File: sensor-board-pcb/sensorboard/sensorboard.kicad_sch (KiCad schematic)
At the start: 138 parts, among them J1 TO_MOTHERBOARD_JACK, J10 PZT_008, J100 PZT_098, J101 PZT_099, J102 PZT_100, J103 PZT_101, J104 PZT_102, J105 PZT_103, J106 PZT_104, J107 PZT_105, J108 PZT_106, J109 PZT_107, J11 PZT_009, J110 PZT_108, J111 PZT_109, J112 PZT_110, J113 PZT_111, J114 PZT_112, J115 PZT_113, J116 PZT_114, J117 PZT_115, J118 PZT_116, J119 PZT_117, J12 PZT_010, J120 PZT_118, J121 PZT_119, J122 PZT_120, J123 PZT_121, J124 PZT_122, J125 PZT_123, J126 PZT_124, J127 PZT_125, J128 PZT_126, J129 PZT_127, J13 PZT_011, J14 PZT_012, J15 PZT_013, J16 PZT_014, J17 PZT_015, J18 PZT_016, J19 PZT_017, J2 PZT_000, J20 PZT_018, J21 PZT_019, J22 PZT_020, J23 PZT_021, J24 PZT_022, J25 PZT_023, J26 PZT_024, J27 PZT_025, J28 PZT_026, J29 PZT_027, J3 PZT_001, J30 PZT_028, J31 PZT_029, J32 PZT_030, J33 PZT_031, J34 PZT_032, J35 PZT_033, J36 PZT_034, J37 PZT_035, J38 PZT_036, J39 PZT_037, J4 PZT_002, J40 PZT_038, J41 PZT_039, J42 PZT_040, J43 PZT_041, J44 PZT_042, J45 PZT_043, J46 PZT_044, J47 PZT_045, J48 PZT_046, J49 PZT_047, J5 PZT_003, J50 PZT_048, J51 PZT_049, J52 PZT_050, J53 PZT_051, J54 PZT_052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

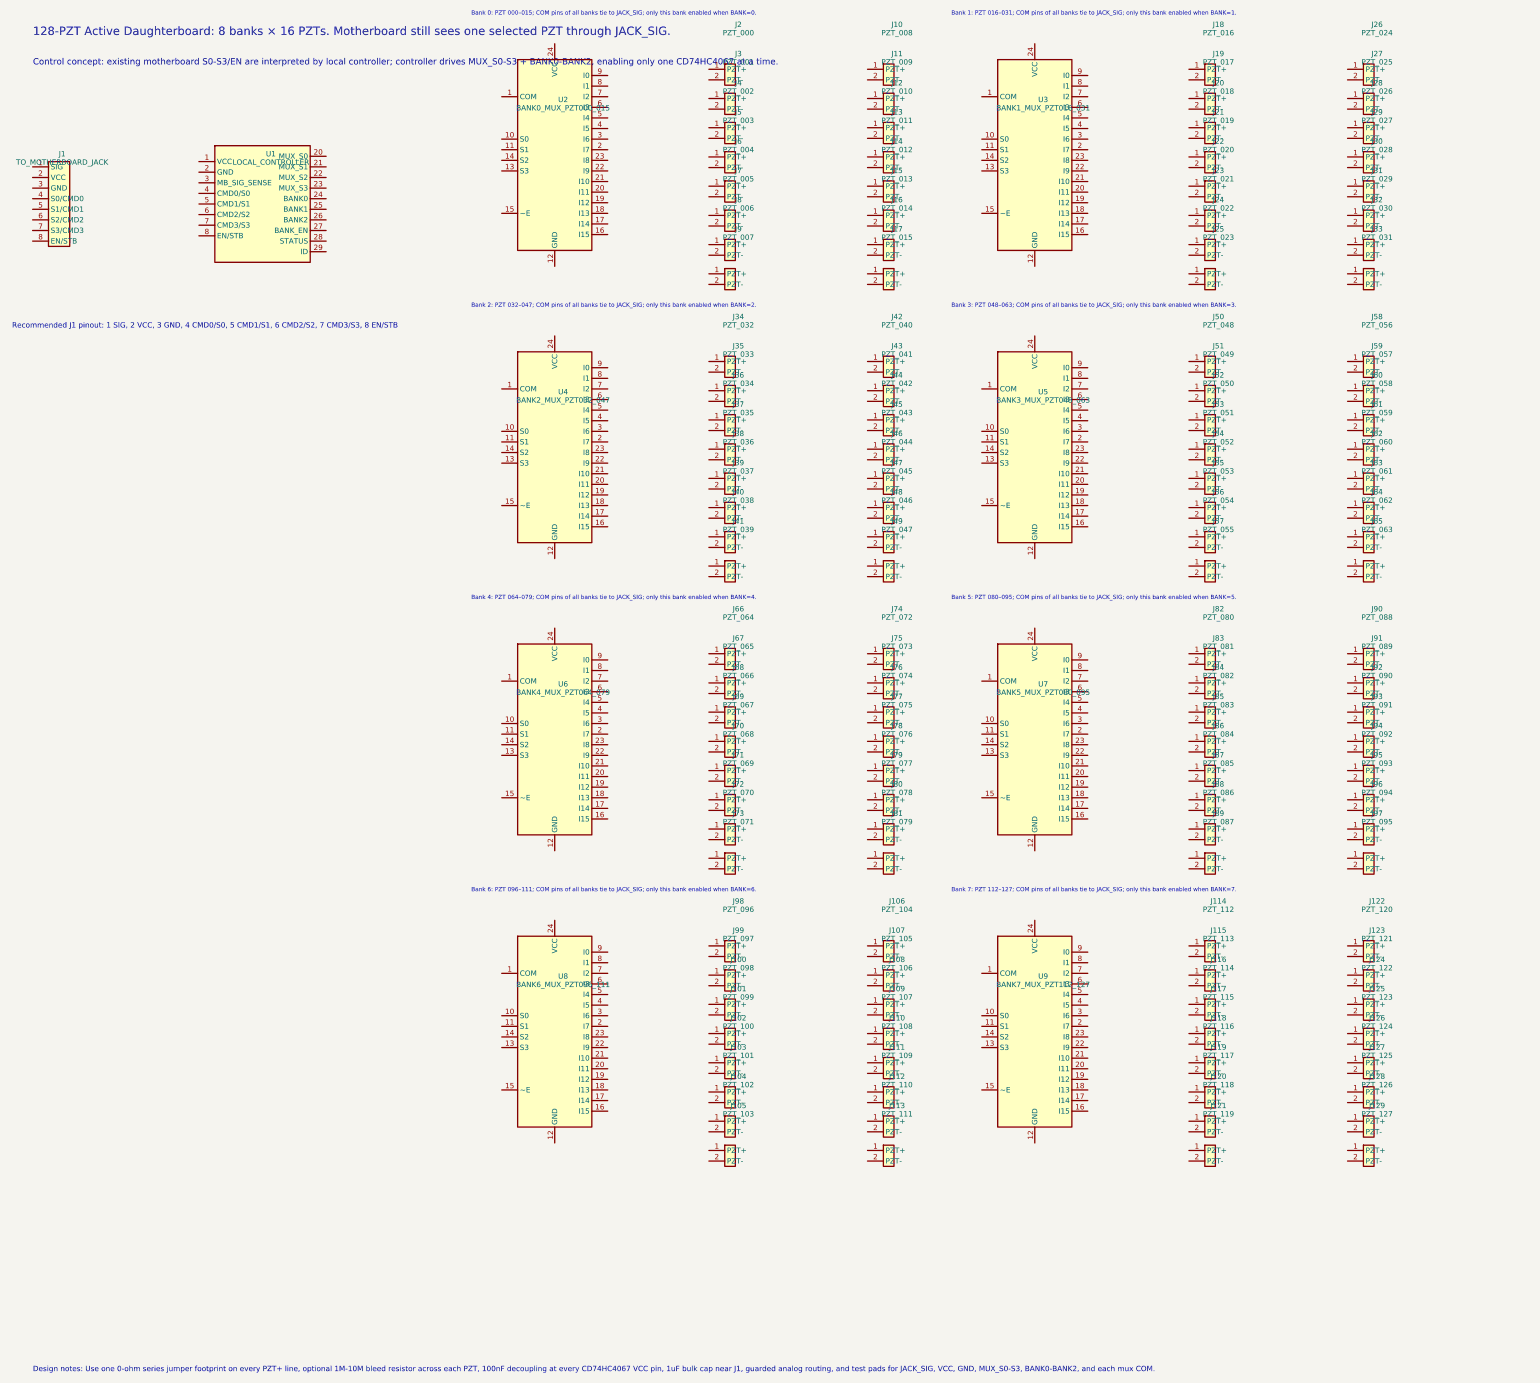
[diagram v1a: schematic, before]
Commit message: fix schem
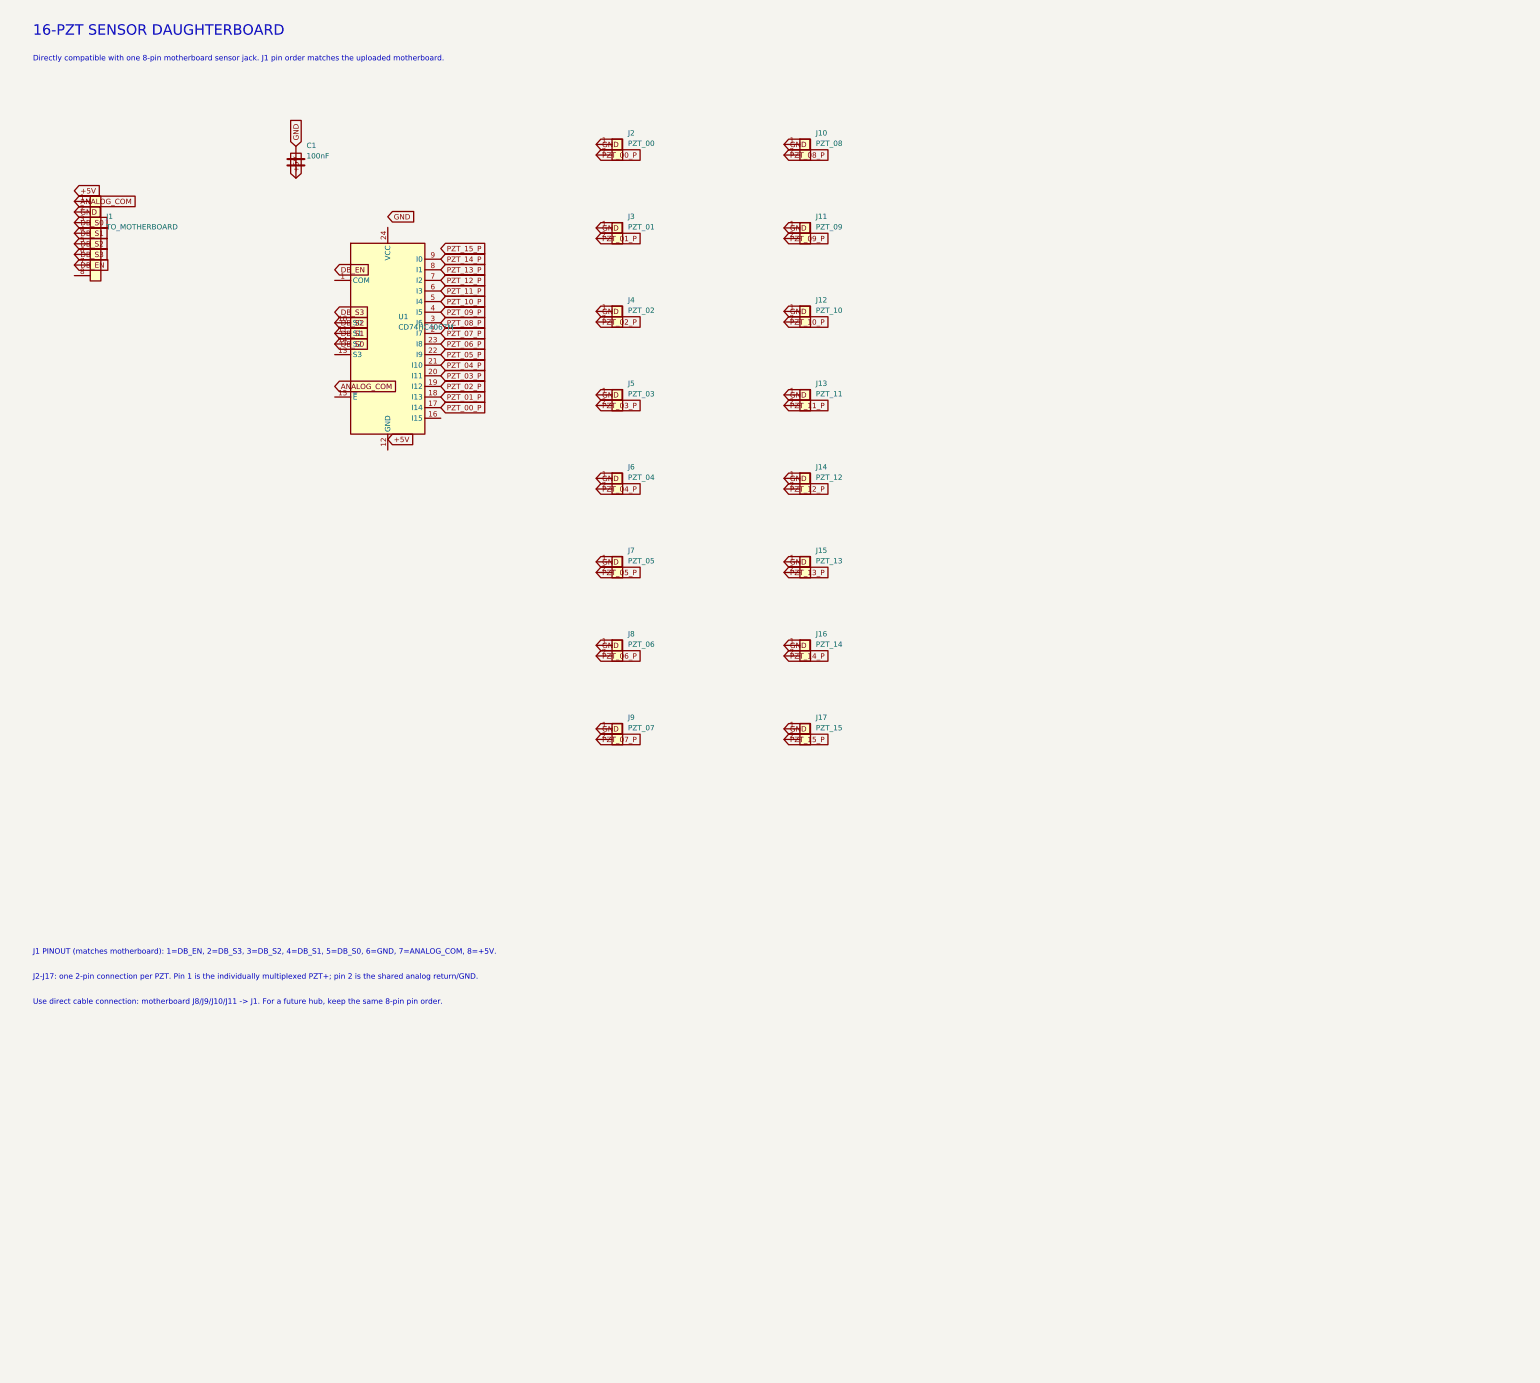
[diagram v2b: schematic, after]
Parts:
- removed J1: TO_MOTHERBOARD_JACK, Connector_PinHeader_2.54mm:PinHeader_1x08_P2.54mm_Vertical, symbol Daughter:MicroFit_01x08_Motherboard
- removed J10: PZT_008, Connector_PinHeader_2.54mm:PinHeader_1x02_P2.54mm_Vertical, symbol Daughter:PZT_Conn_01x02
- removed J100: PZT_098, Connector_PinHeader_2.54mm:PinHeader_1x02_P2.54mm_Vertical, symbol Daughter:PZT_Conn_01x02
- removed J101: PZT_099, Connector_PinHeader_2.54mm:PinHeader_1x02_P2.54mm_Vertical, symbol Daughter:PZT_Conn_01x02
- removed J102: PZT_100, Connector_PinHeader_2.54mm:PinHeader_1x02_P2.54mm_Vertical, symbol Daughter:PZT_Conn_01x02
- removed J103: PZT_101, Connector_PinHeader_2.54mm:PinHeader_1x02_P2.54mm_Vertical, symbol Daughter:PZT_Conn_01x02
- removed J104: PZT_102, Connector_PinHeader_2.54mm:PinHeader_1x02_P2.54mm_Vertical, symbol Daughter:PZT_Conn_01x02
- removed J105: PZT_103, Connector_PinHeader_2.54mm:PinHeader_1x02_P2.54mm_Vertical, symbol Daughter:PZT_Conn_01x02
- removed J106: PZT_104, Connector_PinHeader_2.54mm:PinHeader_1x02_P2.54mm_Vertical, symbol Daughter:PZT_Conn_01x02
- removed J107: PZT_105, Connector_PinHeader_2.54mm:PinHeader_1x02_P2.54mm_Vertical, symbol Daughter:PZT_Conn_01x02
- removed J108: PZT_106, Connector_PinHeader_2.54mm:PinHeader_1x02_P2.54mm_Vertical, symbol Daughter:PZT_Conn_01x02
- removed J109: PZT_107, Connector_PinHeader_2.54mm:PinHeader_1x02_P2.54mm_Vertical, symbol Daughter:PZT_Conn_01x02
- removed J11: PZT_009, Connector_PinHeader_2.54mm:PinHeader_1x02_P2.54mm_Vertical, symbol Daughter:PZT_Conn_01x02
- removed J110: PZT_108, Connector_PinHeader_2.54mm:PinHeader_1x02_P2.54mm_Vertical, symbol Daughter:PZT_Conn_01x02
- removed J111: PZT_109, Connector_PinHeader_2.54mm:PinHeader_1x02_P2.54mm_Vertical, symbol Daughter:PZT_Conn_01x02
- removed J112: PZT_110, Connector_PinHeader_2.54mm:PinHeader_1x02_P2.54mm_Vertical, symbol Daughter:PZT_Conn_01x02
- removed J113: PZT_111, Connector_PinHeader_2.54mm:PinHeader_1x02_P2.54mm_Vertical, symbol Daughter:PZT_Conn_01x02
- removed J114: PZT_112, Connector_PinHeader_2.54mm:PinHeader_1x02_P2.54mm_Vertical, symbol Daughter:PZT_Conn_01x02
- removed J115: PZT_113, Connector_PinHeader_2.54mm:PinHeader_1x02_P2.54mm_Vertical, symbol Daughter:PZT_Conn_01x02
- removed J116: PZT_114, Connector_PinHeader_2.54mm:PinHeader_1x02_P2.54mm_Vertical, symbol Daughter:PZT_Conn_01x02
- removed J117: PZT_115, Connector_PinHeader_2.54mm:PinHeader_1x02_P2.54mm_Vertical, symbol Daughter:PZT_Conn_01x02
- removed J118: PZT_116, Connector_PinHeader_2.54mm:PinHeader_1x02_P2.54mm_Vertical, symbol Daughter:PZT_Conn_01x02
- removed J119: PZT_117, Connector_PinHeader_2.54mm:PinHeader_1x02_P2.54mm_Vertical, symbol Daughter:PZT_Conn_01x02
- removed J12: PZT_010, Connector_PinHeader_2.54mm:PinHeader_1x02_P2.54mm_Vertical, symbol Daughter:PZT_Conn_01x02
- removed J120: PZT_118, Connector_PinHeader_2.54mm:PinHeader_1x02_P2.54mm_Vertical, symbol Daughter:PZT_Conn_01x02
- removed J121: PZT_119, Connector_PinHeader_2.54mm:PinHeader_1x02_P2.54mm_Vertical, symbol Daughter:PZT_Conn_01x02
- removed J122: PZT_120, Connector_PinHeader_2.54mm:PinHeader_1x02_P2.54mm_Vertical, symbol Daughter:PZT_Conn_01x02
- removed J123: PZT_121, Connector_PinHeader_2.54mm:PinHeader_1x02_P2.54mm_Vertical, symbol Daughter:PZT_Conn_01x02
- removed J124: PZT_122, Connector_PinHeader_2.54mm:PinHeader_1x02_P2.54mm_Vertical, symbol Daughter:PZT_Conn_01x02
- removed J125: PZT_123, Connector_PinHeader_2.54mm:PinHeader_1x02_P2.54mm_Vertical, symbol Daughter:PZT_Conn_01x02
- removed J126: PZT_124, Connector_PinHeader_2.54mm:PinHeader_1x02_P2.54mm_Vertical, symbol Daughter:PZT_Conn_01x02
- removed J127: PZT_125, Connector_PinHeader_2.54mm:PinHeader_1x02_P2.54mm_Vertical, symbol Daughter:PZT_Conn_01x02
- removed J128: PZT_126, Connector_PinHeader_2.54mm:PinHeader_1x02_P2.54mm_Vertical, symbol Daughter:PZT_Conn_01x02
- removed J129: PZT_127, Connector_PinHeader_2.54mm:PinHeader_1x02_P2.54mm_Vertical, symbol Daughter:PZT_Conn_01x02
- removed J13: PZT_011, Connector_PinHeader_2.54mm:PinHeader_1x02_P2.54mm_Vertical, symbol Daughter:PZT_Conn_01x02
- removed J14: PZT_012, Connector_PinHeader_2.54mm:PinHeader_1x02_P2.54mm_Vertical, symbol Daughter:PZT_Conn_01x02
- removed J15: PZT_013, Connector_PinHeader_2.54mm:PinHeader_1x02_P2.54mm_Vertical, symbol Daughter:PZT_Conn_01x02
- removed J16: PZT_014, Connector_PinHeader_2.54mm:PinHeader_1x02_P2.54mm_Vertical, symbol Daughter:PZT_Conn_01x02
- removed J17: PZT_015, Connector_PinHeader_2.54mm:PinHeader_1x02_P2.54mm_Vertical, symbol Daughter:PZT_Conn_01x02
- removed J18: PZT_016, Connector_PinHeader_2.54mm:PinHeader_1x02_P2.54mm_Vertical, symbol Daughter:PZT_Conn_01x02
- removed J19: PZT_017, Connector_PinHeader_2.54mm:PinHeader_1x02_P2.54mm_Vertical, symbol Daughter:PZT_Conn_01x02
- removed J2: PZT_000, Connector_PinHeader_2.54mm:PinHeader_1x02_P2.54mm_Vertical, symbol Daughter:PZT_Conn_01x02
- removed J20: PZT_018, Connector_PinHeader_2.54mm:PinHeader_1x02_P2.54mm_Vertical, symbol Daughter:PZT_Conn_01x02
- removed J21: PZT_019, Connector_PinHeader_2.54mm:PinHeader_1x02_P2.54mm_Vertical, symbol Daughter:PZT_Conn_01x02
- removed J22: PZT_020, Connector_PinHeader_2.54mm:PinHeader_1x02_P2.54mm_Vertical, symbol Daughter:PZT_Conn_01x02
- removed J23: PZT_021, Connector_PinHeader_2.54mm:PinHeader_1x02_P2.54mm_Vertical, symbol Daughter:PZT_Conn_01x02
- removed J24: PZT_022, Connector_PinHeader_2.54mm:PinHeader_1x02_P2.54mm_Vertical, symbol Daughter:PZT_Conn_01x02
- removed J25: PZT_023, Connector_PinHeader_2.54mm:PinHeader_1x02_P2.54mm_Vertical, symbol Daughter:PZT_Conn_01x02
- removed J26: PZT_024, Connector_PinHeader_2.54mm:PinHeader_1x02_P2.54mm_Vertical, symbol Daughter:PZT_Conn_01x02
- removed J27: PZT_025, Connector_PinHeader_2.54mm:PinHeader_1x02_P2.54mm_Vertical, symbol Daughter:PZT_Conn_01x02
- removed J28: PZT_026, Connector_PinHeader_2.54mm:PinHeader_1x02_P2.54mm_Vertical, symbol Daughter:PZT_Conn_01x02
- removed J29: PZT_027, Connector_PinHeader_2.54mm:PinHeader_1x02_P2.54mm_Vertical, symbol Daughter:PZT_Conn_01x02
- removed J3: PZT_001, Connector_PinHeader_2.54mm:PinHeader_1x02_P2.54mm_Vertical, symbol Daughter:PZT_Conn_01x02
- removed J30: PZT_028, Connector_PinHeader_2.54mm:PinHeader_1x02_P2.54mm_Vertical, symbol Daughter:PZT_Conn_01x02
- removed J31: PZT_029, Connector_PinHeader_2.54mm:PinHeader_1x02_P2.54mm_Vertical, symbol Daughter:PZT_Conn_01x02
- removed J32: PZT_030, Connector_PinHeader_2.54mm:PinHeader_1x02_P2.54mm_Vertical, symbol Daughter:PZT_Conn_01x02
- removed J33: PZT_031, Connector_PinHeader_2.54mm:PinHeader_1x02_P2.54mm_Vertical, symbol Daughter:PZT_Conn_01x02
- removed J34: PZT_032, Connector_PinHeader_2.54mm:PinHeader_1x02_P2.54mm_Vertical, symbol Daughter:PZT_Conn_01x02
- removed J35: PZT_033, Connector_PinHeader_2.54mm:PinHeader_1x02_P2.54mm_Vertical, symbol Daughter:PZT_Conn_01x02
- removed J36: PZT_034, Connector_PinHeader_2.54mm:PinHeader_1x02_P2.54mm_Vertical, symbol Daughter:PZT_Conn_01x02
- removed J37: PZT_035, Connector_PinHeader_2.54mm:PinHeader_1x02_P2.54mm_Vertical, symbol Daughter:PZT_Conn_01x02
- removed J38: PZT_036, Connector_PinHeader_2.54mm:PinHeader_1x02_P2.54mm_Vertical, symbol Daughter:PZT_Conn_01x02
- removed J39: PZT_037, Connector_PinHeader_2.54mm:PinHeader_1x02_P2.54mm_Vertical, symbol Daughter:PZT_Conn_01x02
- removed J4: PZT_002, Connector_PinHeader_2.54mm:PinHeader_1x02_P2.54mm_Vertical, symbol Daughter:PZT_Conn_01x02
- removed J40: PZT_038, Connector_PinHeader_2.54mm:PinHeader_1x02_P2.54mm_Vertical, symbol Daughter:PZT_Conn_01x02
- removed J41: PZT_039, Connector_PinHeader_2.54mm:PinHeader_1x02_P2.54mm_Vertical, symbol Daughter:PZT_Conn_01x02
- removed J42: PZT_040, Connector_PinHeader_2.54mm:PinHeader_1x02_P2.54mm_Vertical, symbol Daughter:PZT_Conn_01x02
- removed J43: PZT_041, Connector_PinHeader_2.54mm:PinHeader_1x02_P2.54mm_Vertical, symbol Daughter:PZT_Conn_01x02
- removed J44: PZT_042, Connector_PinHeader_2.54mm:PinHeader_1x02_P2.54mm_Vertical, symbol Daughter:PZT_Conn_01x02
- removed J45: PZT_043, Connector_PinHeader_2.54mm:PinHeader_1x02_P2.54mm_Vertical, symbol Daughter:PZT_Conn_01x02
- removed J46: PZT_044, Connector_PinHeader_2.54mm:PinHeader_1x02_P2.54mm_Vertical, symbol Daughter:PZT_Conn_01x02
- removed J47: PZT_045, Connector_PinHeader_2.54mm:PinHeader_1x02_P2.54mm_Vertical, symbol Daughter:PZT_Conn_01x02
- removed J48: PZT_046, Connector_PinHeader_2.54mm:PinHeader_1x02_P2.54mm_Vertical, symbol Daughter:PZT_Conn_01x02
- removed J49: PZT_047, Connector_PinHeader_2.54mm:PinHeader_1x02_P2.54mm_Vertical, symbol Daughter:PZT_Conn_01x02
- removed J5: PZT_003, Connector_PinHeader_2.54mm:PinHeader_1x02_P2.54mm_Vertical, symbol Daughter:PZT_Conn_01x02
- removed J50: PZT_048, Connector_PinHeader_2.54mm:PinHeader_1x02_P2.54mm_Vertical, symbol Daughter:PZT_Conn_01x02
- removed J51: PZT_049, Connector_PinHeader_2.54mm:PinHeader_1x02_P2.54mm_Vertical, symbol Daughter:PZT_Conn_01x02
- removed J52: PZT_050, Connector_PinHeader_2.54mm:PinHeader_1x02_P2.54mm_Vertical, symbol Daughter:PZT_Conn_01x02
- removed J53: PZT_051, Connector_PinHeader_2.54mm:PinHeader_1x02_P2.54mm_Vertical, symbol Daughter:PZT_Conn_01x02
- removed J54: PZT_052, Connector_PinHeader_2.54mm:PinHeader_1x02_P2.54mm_Vertical, symbol Daughter:PZT_Conn_01x02
- removed J55: PZT_053, Connector_PinHeader_2.54mm:PinHeader_1x02_P2.54mm_Vertical, symbol Daughter:PZT_Conn_01x02
- removed J56: PZT_054, Connector_PinHeader_2.54mm:PinHeader_1x02_P2.54mm_Vertical, symbol Daughter:PZT_Conn_01x02
- removed J57: PZT_055, Connector_PinHeader_2.54mm:PinHeader_1x02_P2.54mm_Vertical, symbol Daughter:PZT_Conn_01x02
- removed J58: PZT_056, Connector_PinHeader_2.54mm:PinHeader_1x02_P2.54mm_Vertical, symbol Daughter:PZT_Conn_01x02
- removed J59: PZT_057, Connector_PinHeader_2.54mm:PinHeader_1x02_P2.54mm_Vertical, symbol Daughter:PZT_Conn_01x02
- removed J6: PZT_004, Connector_PinHeader_2.54mm:PinHeader_1x02_P2.54mm_Vertical, symbol Daughter:PZT_Conn_01x02
- removed J60: PZT_058, Connector_PinHeader_2.54mm:PinHeader_1x02_P2.54mm_Vertical, symbol Daughter:PZT_Conn_01x02
- removed J61: PZT_059, Connector_PinHeader_2.54mm:PinHeader_1x02_P2.54mm_Vertical, symbol Daughter:PZT_Conn_01x02
- removed J62: PZT_060, Connector_PinHeader_2.54mm:PinHeader_1x02_P2.54mm_Vertical, symbol Daughter:PZT_Conn_01x02
- removed J63: PZT_061, Connector_PinHeader_2.54mm:PinHeader_1x02_P2.54mm_Vertical, symbol Daughter:PZT_Conn_01x02
- removed J64: PZT_062, Connector_PinHeader_2.54mm:PinHeader_1x02_P2.54mm_Vertical, symbol Daughter:PZT_Conn_01x02
- removed J65: PZT_063, Connector_PinHeader_2.54mm:PinHeader_1x02_P2.54mm_Vertical, symbol Daughter:PZT_Conn_01x02
- removed J66: PZT_064, Connector_PinHeader_2.54mm:PinHeader_1x02_P2.54mm_Vertical, symbol Daughter:PZT_Conn_01x02
- removed J67: PZT_065, Connector_PinHeader_2.54mm:PinHeader_1x02_P2.54mm_Vertical, symbol Daughter:PZT_Conn_01x02
- removed J68: PZT_066, Connector_PinHeader_2.54mm:PinHeader_1x02_P2.54mm_Vertical, symbol Daughter:PZT_Conn_01x02
- removed J69: PZT_067, Connector_PinHeader_2.54mm:PinHeader_1x02_P2.54mm_Vertical, symbol Daughter:PZT_Conn_01x02
- removed J7: PZT_005, Connector_PinHeader_2.54mm:PinHeader_1x02_P2.54mm_Vertical, symbol Daughter:PZT_Conn_01x02
- removed J70: PZT_068, Connector_PinHeader_2.54mm:PinHeader_1x02_P2.54mm_Vertical, symbol Daughter:PZT_Conn_01x02
- removed J71: PZT_069, Connector_PinHeader_2.54mm:PinHeader_1x02_P2.54mm_Vertical, symbol Daughter:PZT_Conn_01x02
- removed J72: PZT_070, Connector_PinHeader_2.54mm:PinHeader_1x02_P2.54mm_Vertical, symbol Daughter:PZT_Conn_01x02
- removed J73: PZT_071, Connector_PinHeader_2.54mm:PinHeader_1x02_P2.54mm_Vertical, symbol Daughter:PZT_Conn_01x02
- removed J74: PZT_072, Connector_PinHeader_2.54mm:PinHeader_1x02_P2.54mm_Vertical, symbol Daughter:PZT_Conn_01x02
- removed J75: PZT_073, Connector_PinHeader_2.54mm:PinHeader_1x02_P2.54mm_Vertical, symbol Daughter:PZT_Conn_01x02
- removed J76: PZT_074, Connector_PinHeader_2.54mm:PinHeader_1x02_P2.54mm_Vertical, symbol Daughter:PZT_Conn_01x02
- removed J77: PZT_075, Connector_PinHeader_2.54mm:PinHeader_1x02_P2.54mm_Vertical, symbol Daughter:PZT_Conn_01x02
- removed J78: PZT_076, Connector_PinHeader_2.54mm:PinHeader_1x02_P2.54mm_Vertical, symbol Daughter:PZT_Conn_01x02
- removed J79: PZT_077, Connector_PinHeader_2.54mm:PinHeader_1x02_P2.54mm_Vertical, symbol Daughter:PZT_Conn_01x02
- removed J8: PZT_006, Connector_PinHeader_2.54mm:PinHeader_1x02_P2.54mm_Vertical, symbol Daughter:PZT_Conn_01x02
- removed J80: PZT_078, Connector_PinHeader_2.54mm:PinHeader_1x02_P2.54mm_Vertical, symbol Daughter:PZT_Conn_01x02
- removed J81: PZT_079, Connector_PinHeader_2.54mm:PinHeader_1x02_P2.54mm_Vertical, symbol Daughter:PZT_Conn_01x02
- removed J82: PZT_080, Connector_PinHeader_2.54mm:PinHeader_1x02_P2.54mm_Vertical, symbol Daughter:PZT_Conn_01x02
- removed J83: PZT_081, Connector_PinHeader_2.54mm:PinHeader_1x02_P2.54mm_Vertical, symbol Daughter:PZT_Conn_01x02
- removed J84: PZT_082, Connector_PinHeader_2.54mm:PinHeader_1x02_P2.54mm_Vertical, symbol Daughter:PZT_Conn_01x02
- removed J85: PZT_083, Connector_PinHeader_2.54mm:PinHeader_1x02_P2.54mm_Vertical, symbol Daughter:PZT_Conn_01x02
- removed J86: PZT_084, Connector_PinHeader_2.54mm:PinHeader_1x02_P2.54mm_Vertical, symbol Daughter:PZT_Conn_01x02
- removed J87: PZT_085, Connector_PinHeader_2.54mm:PinHeader_1x02_P2.54mm_Vertical, symbol Daughter:PZT_Conn_01x02
- removed J88: PZT_086, Connector_PinHeader_2.54mm:PinHeader_1x02_P2.54mm_Vertical, symbol Daughter:PZT_Conn_01x02
- removed J89: PZT_087, Connector_PinHeader_2.54mm:PinHeader_1x02_P2.54mm_Vertical, symbol Daughter:PZT_Conn_01x02
- removed J9: PZT_007, Connector_PinHeader_2.54mm:PinHeader_1x02_P2.54mm_Vertical, symbol Daughter:PZT_Conn_01x02
- removed J90: PZT_088, Connector_PinHeader_2.54mm:PinHeader_1x02_P2.54mm_Vertical, symbol Daughter:PZT_Conn_01x02
- removed J91: PZT_089, Connector_PinHeader_2.54mm:PinHeader_1x02_P2.54mm_Vertical, symbol Daughter:PZT_Conn_01x02
- removed J92: PZT_090, Connector_PinHeader_2.54mm:PinHeader_1x02_P2.54mm_Vertical, symbol Daughter:PZT_Conn_01x02
- removed J93: PZT_091, Connector_PinHeader_2.54mm:PinHeader_1x02_P2.54mm_Vertical, symbol Daughter:PZT_Conn_01x02
- removed J94: PZT_092, Connector_PinHeader_2.54mm:PinHeader_1x02_P2.54mm_Vertical, symbol Daughter:PZT_Conn_01x02
- removed J95: PZT_093, Connector_PinHeader_2.54mm:PinHeader_1x02_P2.54mm_Vertical, symbol Daughter:PZT_Conn_01x02
- removed J96: PZT_094, Connector_PinHeader_2.54mm:PinHeader_1x02_P2.54mm_Vertical, symbol Daughter:PZT_Conn_01x02
- removed J97: PZT_095, Connector_PinHeader_2.54mm:PinHeader_1x02_P2.54mm_Vertical, symbol Daughter:PZT_Conn_01x02
- removed J98: PZT_096, Connector_PinHeader_2.54mm:PinHeader_1x02_P2.54mm_Vertical, symbol Daughter:PZT_Conn_01x02
- removed J99: PZT_097, Connector_PinHeader_2.54mm:PinHeader_1x02_P2.54mm_Vertical, symbol Daughter:PZT_Conn_01x02
- removed U1: LOCAL_CONTROLLER, Package_DIP:DIP-20_W7.62mm, symbol Daughter:Local_Controller_or_GPIO
- removed U2: BANK0_MUX_PZT000_015, Package_SO:SOIC-24W_7.5x15.4mm_P1.27mm, symbol Daughter:CD74HC4067M
- removed U3: BANK1_MUX_PZT016_031, Package_SO:SOIC-24W_7.5x15.4mm_P1.27mm, symbol Daughter:CD74HC4067M
- removed U4: BANK2_MUX_PZT032_047, Package_SO:SOIC-24W_7.5x15.4mm_P1.27mm, symbol Daughter:CD74HC4067M
- removed U5: BANK3_MUX_PZT048_063, Package_SO:SOIC-24W_7.5x15.4mm_P1.27mm, symbol Daughter:CD74HC4067M
- removed U6: BANK4_MUX_PZT064_079, Package_SO:SOIC-24W_7.5x15.4mm_P1.27mm, symbol Daughter:CD74HC4067M
- removed U7: BANK5_MUX_PZT080_095, Package_SO:SOIC-24W_7.5x15.4mm_P1.27mm, symbol Daughter:CD74HC4067M
- removed U8: BANK6_MUX_PZT096_111, Package_SO:SOIC-24W_7.5x15.4mm_P1.27mm, symbol Daughter:CD74HC4067M
- removed U9: BANK7_MUX_PZT112_127, Package_SO:SOIC-24W_7.5x15.4mm_P1.27mm, symbol Daughter:CD74HC4067M
- added C1: 100nF, Capacitor_SMD:C_0603_1608Metric, symbol Device:C
- added J1: TO_MOTHERBOARD, Connector_Molex:Molex_Micro-Fit_3.0_43650-0815_1x08_P3.00mm_Vertical, symbol Connector_Generic:Conn_01x08
- added J10: PZT_08, Connector_PinHeader_2.54mm:PinHeader_1x02_P2.54mm_Vertical, symbol Connector_Generic:Conn_01x02
- added J11: PZT_09, Connector_PinHeader_2.54mm:PinHeader_1x02_P2.54mm_Vertical, symbol Connector_Generic:Conn_01x02
- added J12: PZT_10, Connector_PinHeader_2.54mm:PinHeader_1x02_P2.54mm_Vertical, symbol Connector_Generic:Conn_01x02
- added J13: PZT_11, Connector_PinHeader_2.54mm:PinHeader_1x02_P2.54mm_Vertical, symbol Connector_Generic:Conn_01x02
- added J14: PZT_12, Connector_PinHeader_2.54mm:PinHeader_1x02_P2.54mm_Vertical, symbol Connector_Generic:Conn_01x02
- added J15: PZT_13, Connector_PinHeader_2.54mm:PinHeader_1x02_P2.54mm_Vertical, symbol Connector_Generic:Conn_01x02
- added J16: PZT_14, Connector_PinHeader_2.54mm:PinHeader_1x02_P2.54mm_Vertical, symbol Connector_Generic:Conn_01x02
- added J17: PZT_15, Connector_PinHeader_2.54mm:PinHeader_1x02_P2.54mm_Vertical, symbol Connector_Generic:Conn_01x02
- added J2: PZT_00, Connector_PinHeader_2.54mm:PinHeader_1x02_P2.54mm_Vertical, symbol Connector_Generic:Conn_01x02
- added J3: PZT_01, Connector_PinHeader_2.54mm:PinHeader_1x02_P2.54mm_Vertical, symbol Connector_Generic:Conn_01x02
- added J4: PZT_02, Connector_PinHeader_2.54mm:PinHeader_1x02_P2.54mm_Vertical, symbol Connector_Generic:Conn_01x02
- added J5: PZT_03, Connector_PinHeader_2.54mm:PinHeader_1x02_P2.54mm_Vertical, symbol Connector_Generic:Conn_01x02
- added J6: PZT_04, Connector_PinHeader_2.54mm:PinHeader_1x02_P2.54mm_Vertical, symbol Connector_Generic:Conn_01x02
- added J7: PZT_05, Connector_PinHeader_2.54mm:PinHeader_1x02_P2.54mm_Vertical, symbol Connector_Generic:Conn_01x02
- added J8: PZT_06, Connector_PinHeader_2.54mm:PinHeader_1x02_P2.54mm_Vertical, symbol Connector_Generic:Conn_01x02
- added J9: PZT_07, Connector_PinHeader_2.54mm:PinHeader_1x02_P2.54mm_Vertical, symbol Connector_Generic:Conn_01x02
- added U1: CD74HC4067M, Package_SO:SOIC-24W_7.5x15.4mm_P1.27mm, symbol 74xx:CD74HC4067M
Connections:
- new net +5V: C1.2
- new net ANALOG_COM: J1.1 (Pin_1)
- new net DB_EN: J1.7 (Pin_7)
- new net DB_S0: J1.3 (Pin_3), U1.14 (S2)
- new net DB_S1: J1.4 (Pin_4), U1.11 (S1)
- new net DB_S2: J1.5 (Pin_5), U1.10 (S0)
- new net DB_S3: J1.6 (Pin_6)
- new net GND: C1.1, J1.2 (Pin_2), J10.1 (PZT+), J11.1 (PZT+), J12.1 (PZT+), J13.1 (PZT+), J14.1 (PZT+), J15.1 (PZT+), J16.1 (PZT+), J17.1 (PZT+), J2.1 (PZT+), J3.1 (PZT+), J4.1 (PZT+), J5.1 (PZT+), J6.1 (PZT+), J7.1 (PZT+), J8.1 (PZT+), J9.1 (PZT+)
- new net PZT_00_P: J2.2 (PZT-), U1.17 (I14)
- new net PZT_01_P: J3.2 (PZT-), U1.18 (I13)
- new net PZT_02_P: J4.2 (PZT-), U1.19 (I12)
- new net PZT_03_P: J5.2 (PZT-), U1.20 (I11)
- new net PZT_04_P: J6.2 (PZT-), U1.21 (I10)
- new net PZT_05_P: J7.2 (PZT-), U1.22 (I9)
- new net PZT_06_P: J8.2 (PZT-), U1.23 (I8)
- new net PZT_07_P: J9.2 (PZT-), U1.2 (I7)
- new net PZT_08_P: J10.2 (PZT-), U1.3 (I6)
- new net PZT_09_P: J11.2 (PZT-), U1.4 (I5)
- new net PZT_10_P: J12.2 (PZT-), U1.5 (I4)
- new net PZT_11_P: J13.2 (PZT-), U1.6 (I3)
- new net PZT_12_P: J14.2 (PZT-), U1.7 (I2)
- new net PZT_13_P: J15.2 (PZT-), U1.8 (I1)
- new net PZT_14_P: J16.2 (PZT-), U1.9 (I0)
- new net PZT_15_P: J17.2 (PZT-)
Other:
- note added: "16-PZT SENSOR DAUGHTERBOARD"
- note added: "Directly compatible with one 8-pin motherboard sensor jack. J1 pin order matches the uploaded motherboard."
- note added: "J1 PINOUT (matches motherboard): 1=DB_EN, 2=DB_S3, 3=DB_S2, 4=DB_S1, 5=DB_S0, 6=GND, 7=ANALOG_COM, 8=+5V."
- note added: "J2-J17: one 2-pin connection per PZT. Pin 1 is the individually multiplexed PZT+; pin 2 is the shared analog return/GND."
- note added: "Use direct cable connection: motherboard J8/J9/J10/J11 -> J1. For a future hub, keep the same 8-pin pin order."
- note removed: "128-PZT Active Daughterboard: 8 banks × 16 PZTs. Motherboard still sees one selected PZT through JACK_SIG."
- note removed: "Bank 0: PZT 000–015; COM pins of all banks tie to JACK_SIG; only this bank enabled when BANK=0."
- note removed: "Bank 1: PZT 016–031; COM pins of all banks tie to JACK_SIG; only this bank enabled when BANK=1."
- note removed: "Bank 2: PZT 032–047; COM pins of all banks tie to JACK_SIG; only this bank enabled when BANK=2."
- note removed: "Bank 3: PZT 048–063; COM pins of all banks tie to JACK_SIG; only this bank enabled when BANK=3."
- note removed: "Bank 4: PZT 064–079; COM pins of all banks tie to JACK_SIG; only this bank enabled when BANK=4."
- note removed: "Bank 5: PZT 080–095; COM pins of all banks tie to JACK_SIG; only this bank enabled when BANK=5."
- note removed: "Bank 6: PZT 096–111; COM pins of all banks tie to JACK_SIG; only this bank enabled when BANK=6."
- note removed: "Bank 7: PZT 112–127; COM pins of all banks tie to JACK_SIG; only this bank enabled when BANK=7."
- note removed: "Control concept: existing motherboard S0-S3/EN are interpreted by local controller; controller drives MUX_S0-S3 + BANK0-BANK2, enabling only one CD74HC4067 at a time."
- note removed: "Design notes: Use one 0-ohm series jumper footprint on every PZT+ line, optional 1M-10M bleed resistor across each PZT, 100nF decoupling at every CD74HC4067 VCC pin, 1uF bulk cap near J1, guarded analog routing, and test pads for JACK_SIG, VCC, GND, MUX_S0-S3, BANK0-BANK2, and each mux COM."
- note removed: "Recommended J1 pinout: 1 SIG, 2 VCC, 3 GND, 4 CMD0/S0, 5 CMD1/S1, 6 CMD2/S2, 7 CMD3/S3, 8 EN/STB"
